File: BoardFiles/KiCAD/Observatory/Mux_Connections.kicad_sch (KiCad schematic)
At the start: 6 parts, among them U2 Scope 1 Mux, U3 Wave Gen. Mux, U4 Scope 2 Mux

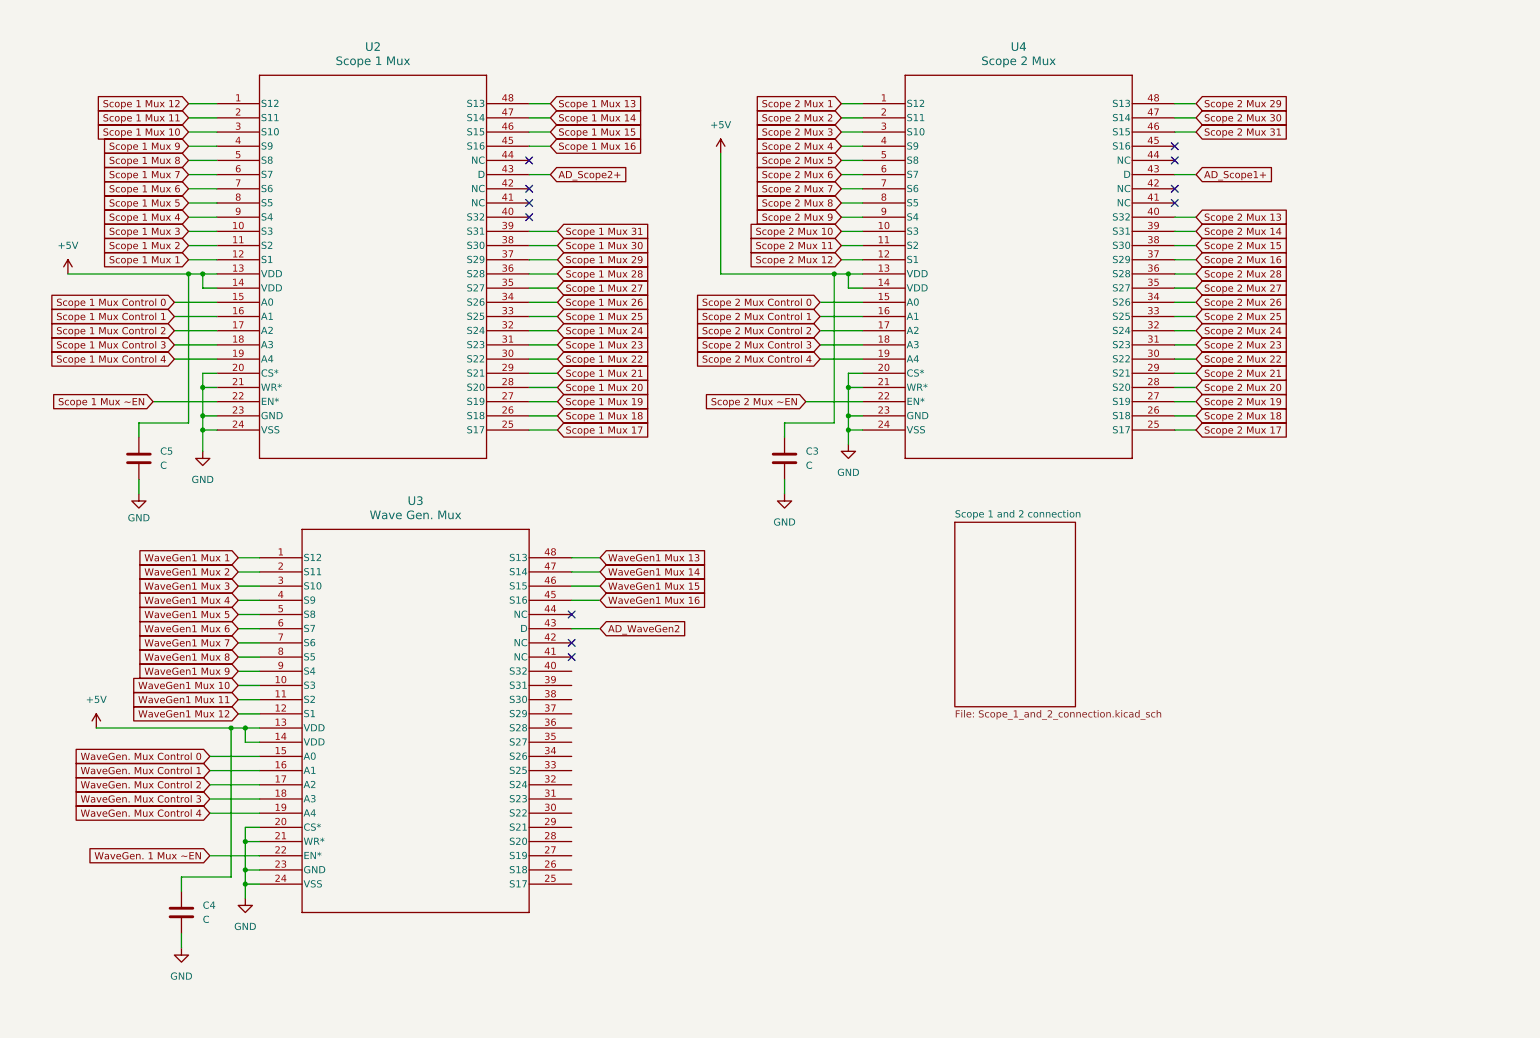
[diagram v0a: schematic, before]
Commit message: REV3 DRC pass
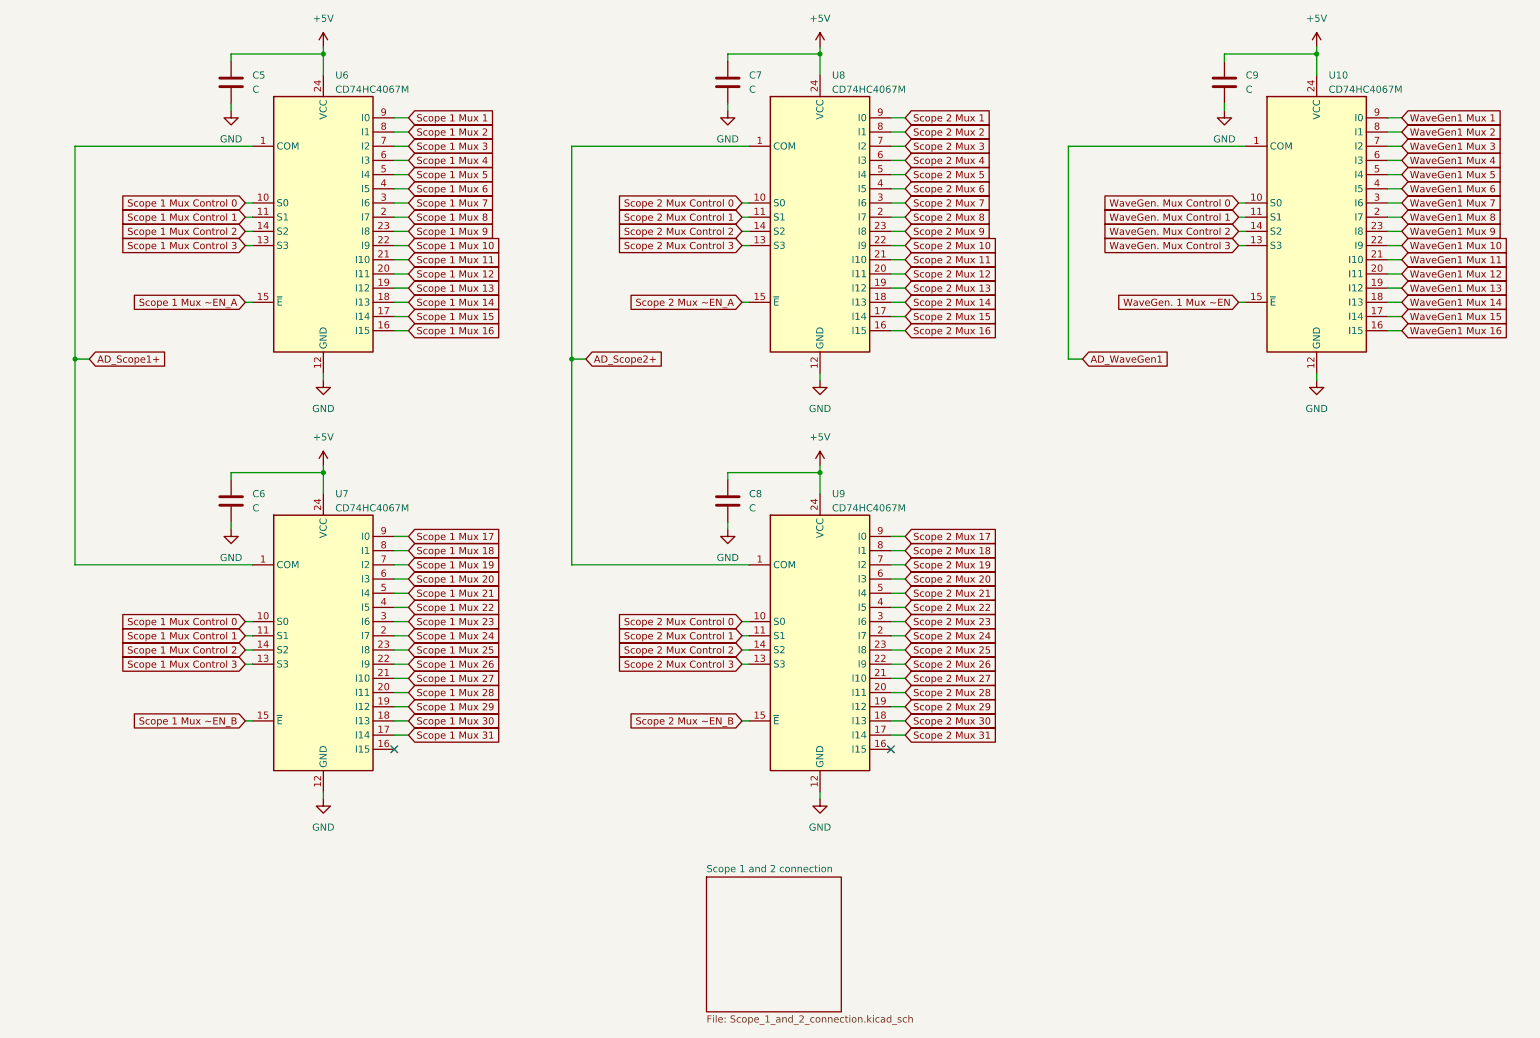
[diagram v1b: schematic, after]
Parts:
- removed C3, C4: C, Capacitor_SMD:C_0805_2012Metric_Pad1.18x1.45mm_HandSolder, symbol Device:C
- removed U2: Scope 1 Mux, SU_48_ADI, symbol 3rdPrty_Symbols:ADG732BSUZ
- removed U3: Wave Gen. Mux, SU_48_ADI, symbol 3rdPrty_Symbols:ADG732BSUZ
- removed U4: Scope 2 Mux, SU_48_ADI, symbol 3rdPrty_Symbols:ADG732BSUZ
- added C6, C7, C8, C9: C, Capacitor_SMD:C_0805_2012Metric_Pad1.18x1.45mm_HandSolder, symbol Device:C
- added U10, U6, U7, U8, U9: CD74HC4067M, Package_SO:SOIC-24W_7.5x15.4mm_P1.27mm, symbol 74xx:CD74HC4067M
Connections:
- net +5V: now also C6.1, C7.1, C8.1, C9.1, U10.24 (VCC), U6.24 (VCC), U7.24 (VCC), U8.24 (VCC), U9.24 (VCC)
- net AD_Scope1+: now also U6.1 (COM), U7.1 (COM)
- net AD_Scope2+: now also U8.1 (COM), U9.1 (COM)
- net GND: now also C6.2, C7.2, C8.2, C9.2, U10.12 (GND), U6.12 (GND), U7.12 (GND), U8.12 (GND), U9.12 (GND)
- net Scope 1 Mux  1: now also U6.9 (I0)
- net Scope 1 Mux  10: now also U6.22 (I9)
- net Scope 1 Mux  11: now also U6.21 (I10)
- net Scope 1 Mux  12: now also U6.20 (I11)
- net Scope 1 Mux  13: now also U6.19 (I12)
- net Scope 1 Mux  14: now also U6.18 (I13)
- net Scope 1 Mux  15: now also U6.17 (I14)
- net Scope 1 Mux  16: now also U6.16 (I15)
- net Scope 1 Mux  17: now also U7.9 (I0)
- net Scope 1 Mux  18: now also U7.8 (I1)
- net Scope 1 Mux  19: now also U7.7 (I2)
- net Scope 1 Mux  2: now also U6.8 (I1)
- net Scope 1 Mux  20: now also U7.6 (I3)
- net Scope 1 Mux  21: now also U7.5 (I4)
- net Scope 1 Mux  22: now also U7.4 (I5)
- net Scope 1 Mux  23: now also U7.3 (I6)
- net Scope 1 Mux  24: now also U7.2 (I7)
- net Scope 1 Mux  25: now also U7.23 (I8)
- net Scope 1 Mux  26: now also U7.22 (I9)
- net Scope 1 Mux  27: now also U7.21 (I10)
- net Scope 1 Mux  28: now also U7.20 (I11)
- net Scope 1 Mux  29: now also U7.19 (I12)
- net Scope 1 Mux  3: now also U6.7 (I2)
- net Scope 1 Mux  30: now also U7.18 (I13)
- net Scope 1 Mux  31: now also U7.17 (I14)
- net Scope 1 Mux  4: now also U6.6 (I3)
- net Scope 1 Mux  5: now also U6.5 (I4)
- net Scope 1 Mux  6: now also U6.4 (I5)
- net Scope 1 Mux  7: now also U6.3 (I6)
- net Scope 1 Mux  8: now also U6.2 (I7)
- net Scope 1 Mux  9: now also U6.23 (I8)
- net Scope 1 Mux Control 0: now also U6.10 (S0), U7.10 (S0)
- net Scope 1 Mux Control 1: now also U6.11 (S1), U7.11 (S1)
- net Scope 1 Mux Control 2: now also U6.14 (S2), U7.14 (S2)
- net Scope 1 Mux Control 3: now also U6.13 (S3), U7.13 (S3)
- net Scope 2 Mux  1: now also U8.9 (I0)
- net Scope 2 Mux  10: now also U8.22 (I9)
- net Scope 2 Mux  11: now also U8.21 (I10)
- net Scope 2 Mux  12: now also U8.20 (I11)
- net Scope 2 Mux  13: now also U8.19 (I12)
- net Scope 2 Mux  14: now also U8.18 (I13)
- net Scope 2 Mux  15: now also U8.17 (I14)
- net Scope 2 Mux  16: now also U8.16 (I15)
- net Scope 2 Mux  17: now also U9.9 (I0)
- net Scope 2 Mux  18: now also U9.8 (I1)
- net Scope 2 Mux  19: now also U9.7 (I2)
- net Scope 2 Mux  2: now also U8.8 (I1)
- net Scope 2 Mux  20: now also U9.6 (I3)
- net Scope 2 Mux  21: now also U9.5 (I4)
- net Scope 2 Mux  22: now also U9.4 (I5)
- net Scope 2 Mux  23: now also U9.3 (I6)
- net Scope 2 Mux  24: now also U9.2 (I7)
- net Scope 2 Mux  25: now also U9.23 (I8)
- net Scope 2 Mux  26: now also U9.22 (I9)
- net Scope 2 Mux  27: now also U9.21 (I10)
- net Scope 2 Mux  28: now also U9.20 (I11)
- net Scope 2 Mux  29: now also U9.19 (I12)
- net Scope 2 Mux  3: now also U8.7 (I2)
- net Scope 2 Mux  30: now also U9.18 (I13)
- net Scope 2 Mux  31: now also U9.17 (I14)
- net Scope 2 Mux  4: now also U8.6 (I3)
- net Scope 2 Mux  5: now also U8.5 (I4)
- net Scope 2 Mux  6: now also U8.4 (I5)
- net Scope 2 Mux  7: now also U8.3 (I6)
- net Scope 2 Mux  8: now also U8.2 (I7)
- net Scope 2 Mux  9: now also U8.23 (I8)
- net Scope 2 Mux Control 0: now also U8.10 (S0), U9.10 (S0)
- net Scope 2 Mux Control 1: now also U8.11 (S1), U9.11 (S1)
- net Scope 2 Mux Control 2: now also U8.14 (S2), U9.14 (S2)
- net Scope 2 Mux Control 3: now also U8.13 (S3), U9.13 (S3)
- net WaveGen. 1 Mux ~EN: now also U10.15 (~{E})
- net WaveGen. Mux Control 0: now also U10.10 (S0)
- net WaveGen. Mux Control 1: now also U10.11 (S1)
- net WaveGen. Mux Control 2: now also U10.14 (S2)
- net WaveGen. Mux Control 3: now also U10.13 (S3)
- net WaveGen1 Mux  1: now also U10.9 (I0)
- net WaveGen1 Mux  10: now also U10.22 (I9)
- net WaveGen1 Mux  11: now also U10.21 (I10)
- net WaveGen1 Mux  12: now also U10.20 (I11)
- net WaveGen1 Mux  13: now also U10.19 (I12)
- net WaveGen1 Mux  14: now also U10.18 (I13)
- net WaveGen1 Mux  15: now also U10.17 (I14)
- net WaveGen1 Mux  16: now also U10.16 (I15)
- net WaveGen1 Mux  2: now also U10.8 (I1)
- net WaveGen1 Mux  3: now also U10.7 (I2)
- net WaveGen1 Mux  4: now also U10.6 (I3)
- net WaveGen1 Mux  5: now also U10.5 (I4)
- net WaveGen1 Mux  6: now also U10.4 (I5)
- net WaveGen1 Mux  7: now also U10.3 (I6)
- net WaveGen1 Mux  8: now also U10.2 (I7)
- net WaveGen1 Mux  9: now also U10.23 (I8)
- new net AD_WaveGen1: U10.1 (COM)
- new net Scope 1 Mux ~EN_A: U6.15 (~{E})
- new net Scope 1 Mux ~EN_B: U7.15 (~{E})
- new net Scope 2 Mux ~EN_A: U8.15 (~{E})
- new net Scope 2 Mux ~EN_B: U9.15 (~{E})
- no-connect marks 11 -> 2
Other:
- moved on the sheet: C5
